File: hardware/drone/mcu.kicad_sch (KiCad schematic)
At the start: 13 parts, among them SW1 SW_MEC_5E, U1 STM32N645I0, U6 MX25UW25645GXDI00

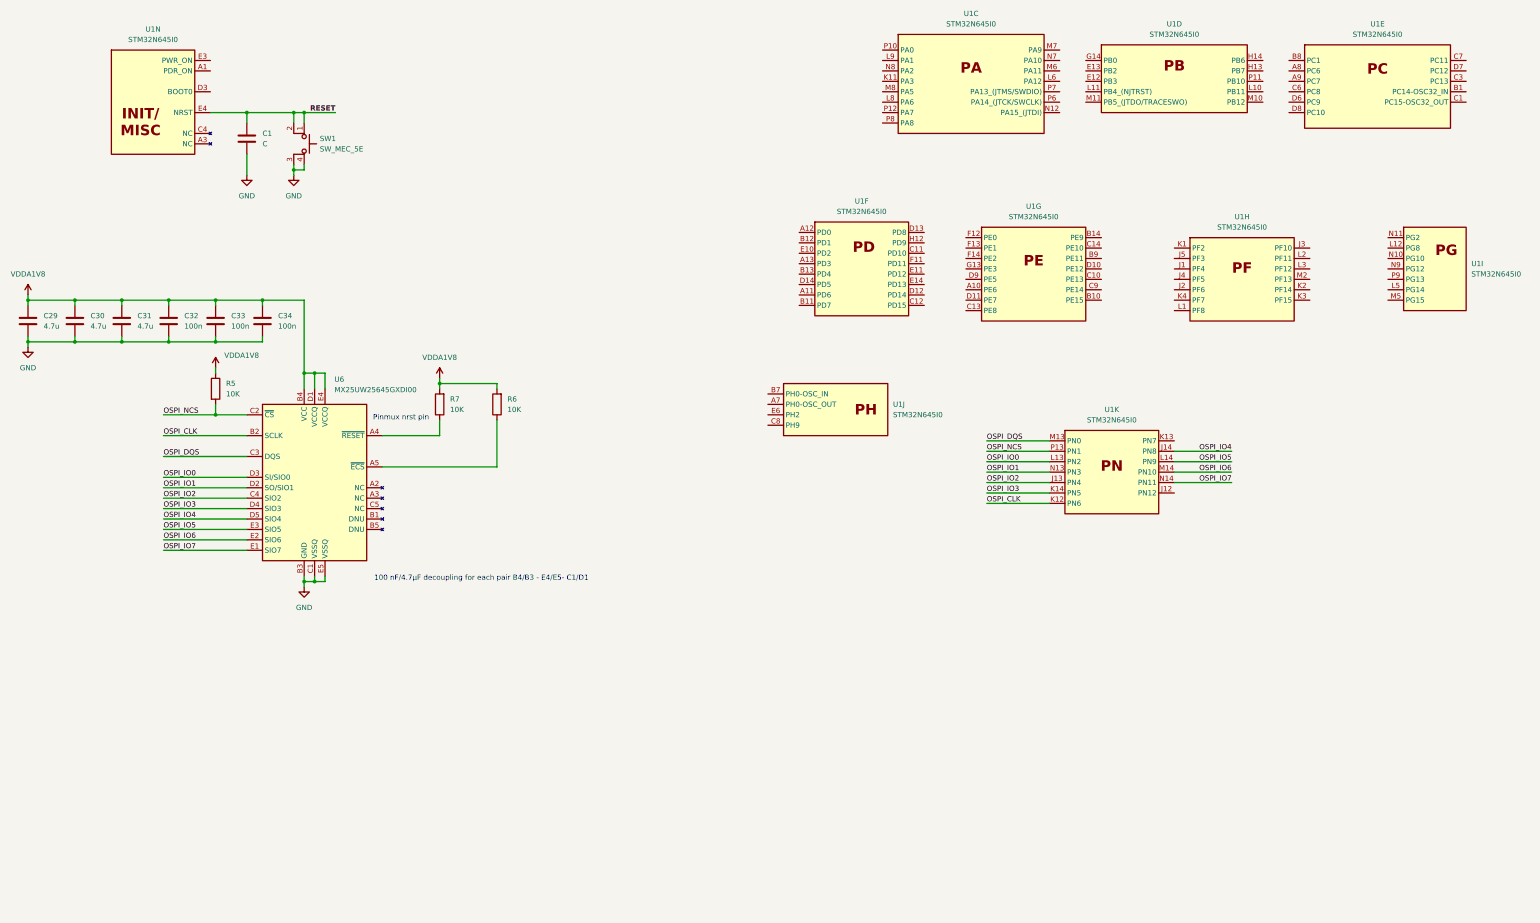
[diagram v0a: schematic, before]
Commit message: more radio work
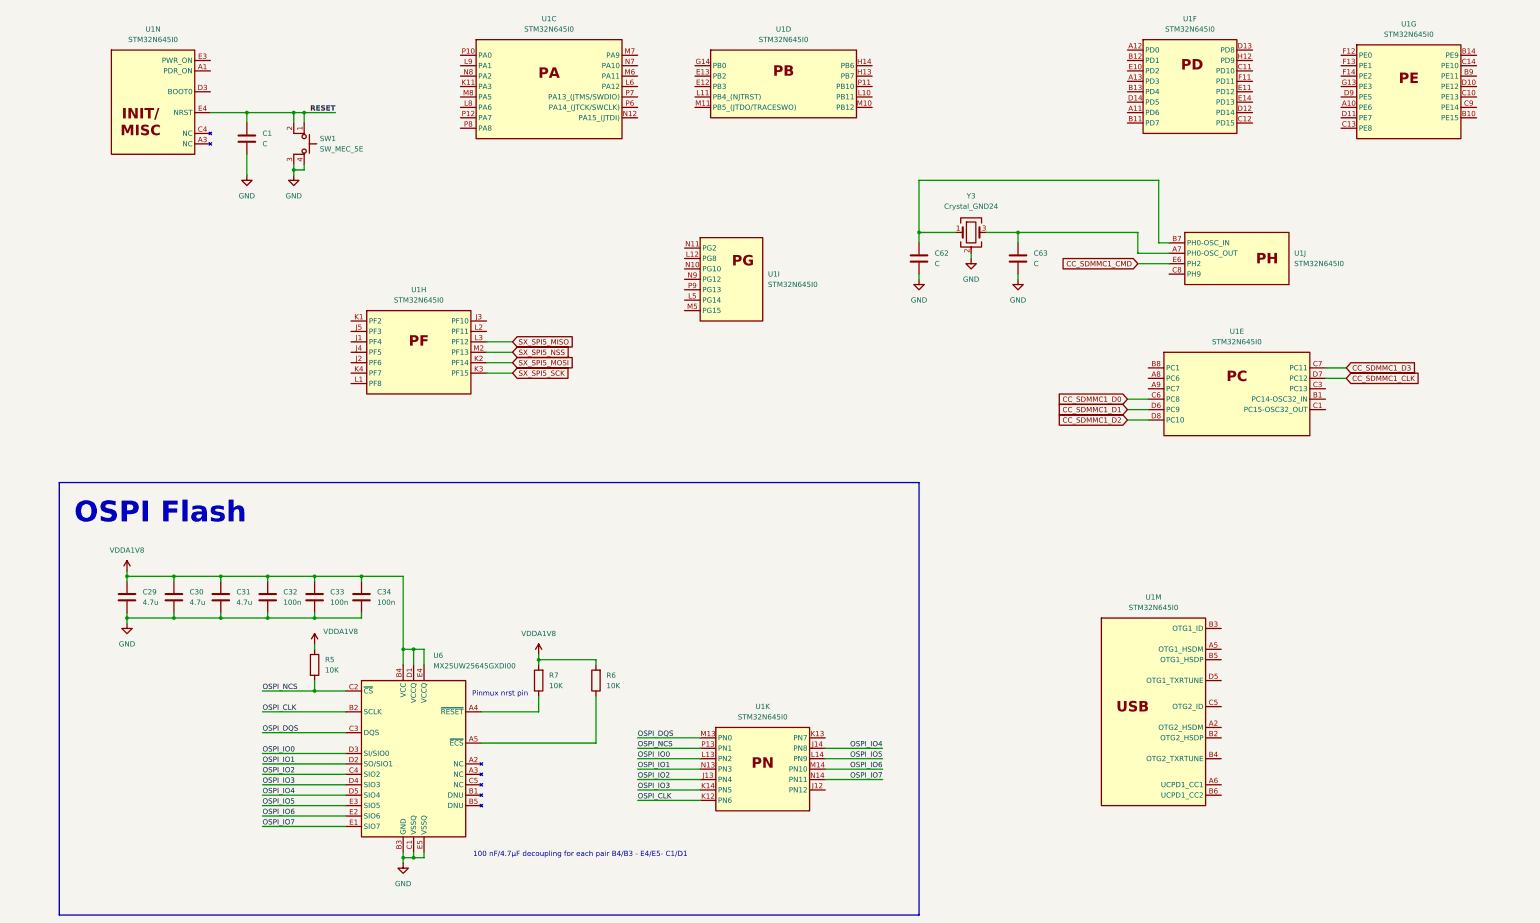
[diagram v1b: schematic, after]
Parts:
- added C62, C63: C, symbol Device:C
- added unit 13 of U1
- added Y3: Crystal_GND24, symbol Device:Crystal_GND24
- U1: footprint STM32N645I0:BGA178C80P14X14_1200X1200X100 -> (none)
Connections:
- net GND: now also C62.2, C63.2, Y3.2 (G), Y3.4 (G)
- net SX_SPI5_MOSI: now reaches U1.K2 (PF14)
- net SX_SPI5_SCK: now reaches U1.K3 (PF15)
- net SX_SPI5_MISO: now reaches U1.L3 (PF12)
- net SX_SPI5_NSS: now reaches U1.M2 (PF13)
- net CC_SDMMC1_D0: now reaches U1.C6 (PC8)
- net CC_SDMMC1_D3: now reaches U1.C7 (PC11)
- net CC_SDMMC1_D1: now reaches U1.D6 (PC9)
- net CC_SDMMC1_CLK: now reaches U1.D7 (PC12)
- net CC_SDMMC1_D2: now reaches U1.D8 (PC10)
- net at U1.A7 (PH0-OSC_OUT): now also C63.1, Y3.3
- net at U1.B7 (PH0-OSC_IN): now also C62.1, Y3.1
- net CC_SDMMC1_CMD: now reaches U1.E6 (PH2)
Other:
- note added: "OSPI Flash"
- moved on the sheet: C29, C30, C31, C32, C33, C34, R5, R6, R7, U6
